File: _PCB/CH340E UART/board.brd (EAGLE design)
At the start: 24.9 x 16.3 mm, 11 parts, among them IC1 REG1117, U1 CH340ESMD

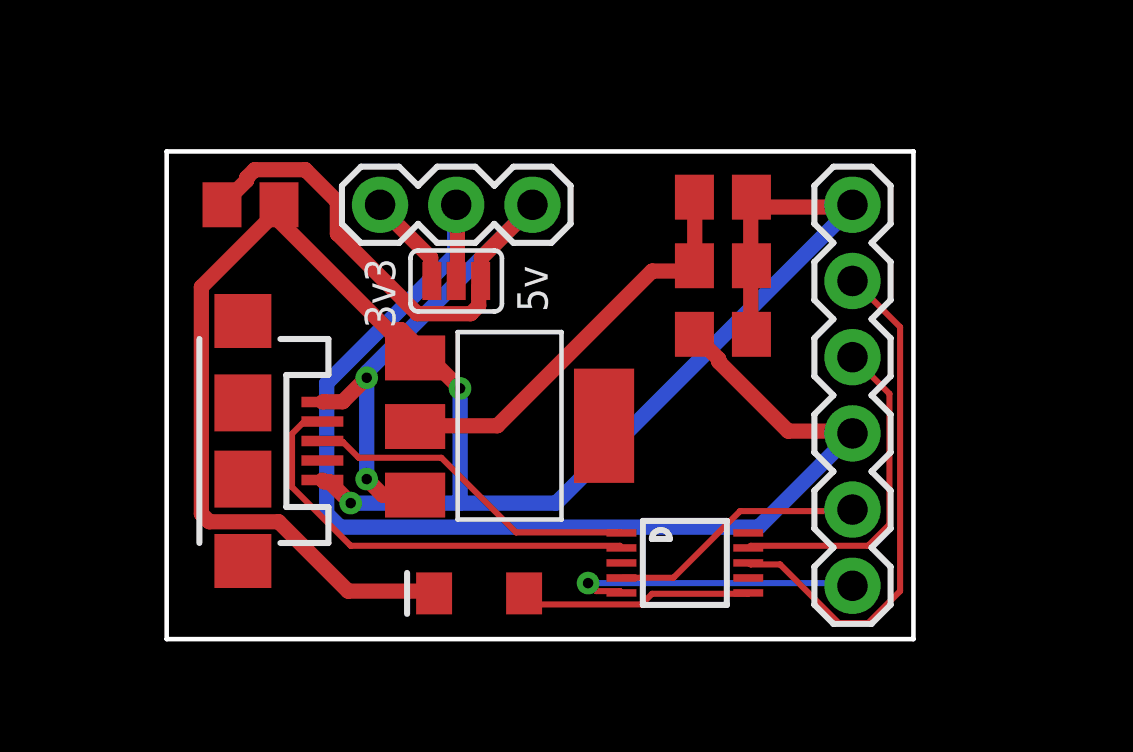
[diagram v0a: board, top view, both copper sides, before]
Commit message: CH340e design complete
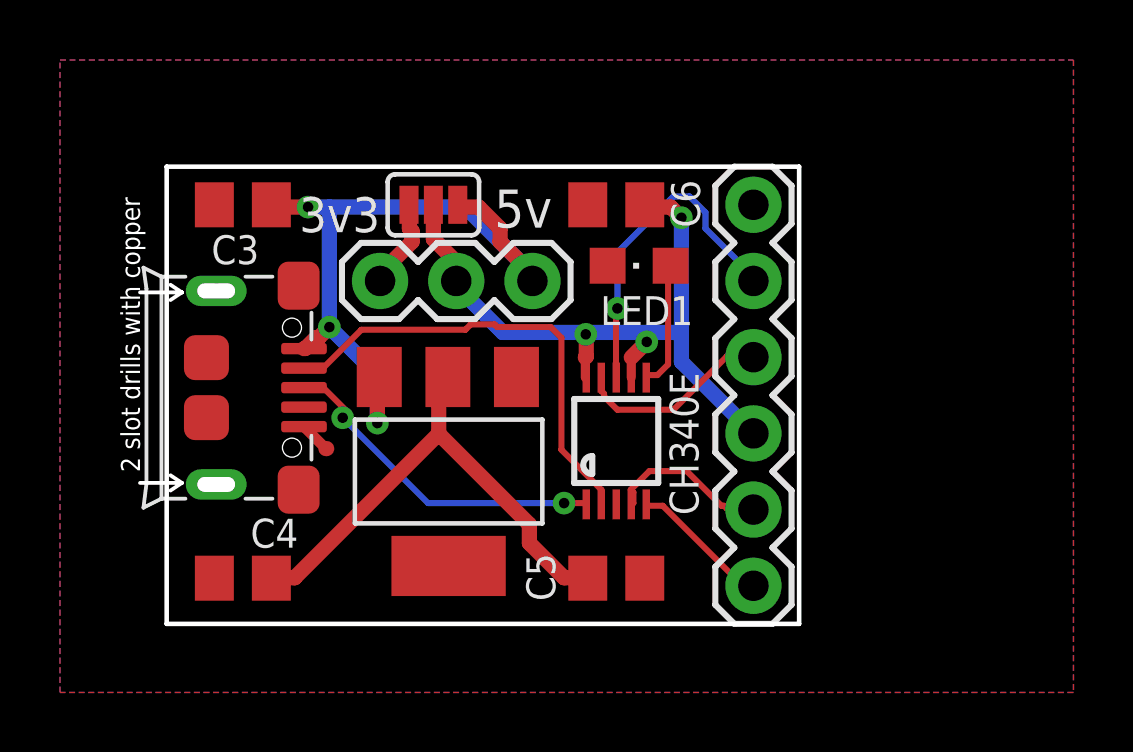
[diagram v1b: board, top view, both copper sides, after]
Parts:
- removed D1: 1206size, SparkFun-LED:LED-1206
- removed J1: (no value), SparkFun-Connectors:USB-MICROB
- removed U1: CH340ESMD, CH340E:MSOP10
- added CH340E: CH340ESMD, CH340E:MSOP10
- added LED1: (no value), adafruit:CHIPLED_0805
- added USB2: ST-USB-001G, Seeed-Connector:MICRO-USB5+4P-SMD-0.65-B
- JP1: device SparkFun-Jumpers:SMT-JUMPER_3_1-NC_PASTE_SILK -> SparkFun-Jumpers:SMT-JUMPER_3_NO_SILK
- moved C4 19.1 mm to (2.54, 2.03), turned to 180 degrees
- moved C5 13.2 mm to (15.0, 2.03)
- moved C6 5.59 mm to (15.0, 14.5), turned to 180 degrees
- moved J2 3.30 mm to (19.6, 1.78)
- moved JP1 2.65 mm to (8.89, 14.5)
- moved IC1 2.54 mm to (9.40, 5.59), turned to 180 degrees
- moved J3 2.54 mm to (12.2, 11.9)
- moved C3 0.25 mm to (2.54, 14.5), turned to 180 degrees
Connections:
- net 5V1 renamed 3V3
- net 5V: now also USB2.1; no longer J1.VBUS
- net CTS: now also CH340E.5; no longer U1.5
- net GND: now also CH340E.3, LED1.C, USB2.5, USB2.S1, USB2.S2, USB2.S3, USB2.S4, USB2.S5, USB2.S6; no longer D1.C, J1.GND, U1.3
- net N$1: now also CH340E.6, LED1.A; no longer D1.A, U1.6
- net RTS: now also CH340E.4; no longer U1.4
- net RX: now also CH340E.9; no longer U1.9
- net TX: now also CH340E.8; no longer U1.8
- net USBN: now also CH340E.2, USB2.2; no longer J1.D-, U1.2
- net USBP: now also CH340E.1, USB2.3; no longer J1.D+, U1.1
- net VCC: now also CH340E.10, CH340E.7; no longer U1.10, U1.7
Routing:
- net GND: track 64.6 -> 1.06 mm, vias 2 -> 0
- net VCC: track 40.4 -> 24.0 mm, vias 0 -> 3
- net 5V: track 31.0 -> 24.4 mm, vias 2 -> 3
- net TX: track 17.3 -> 11.1 mm, vias 0 -> 1
- net CTS: track 10.1 -> 4.71 mm, vias 1 -> 0
- net RX: track 11.1 -> 6.59 mm
- net N$1: track 7.79 -> 4.32 mm
- net RTS: track 8.66 -> 5.47 mm
- net 3V3: track 13.8 -> 16.9 mm
- net USBN: track 14.8 -> 15.5 mm
- net USBP: track 11.2 -> 11.3 mm, vias 0 -> 2
- added copper zone on layer 1, net GND
- added copper zone on layer 16, net GND
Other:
- board size 24.9 x 16.3 mm -> 21.1 x 15.2 mm
- board text added: "CTS"
- board text added: "GND"
- board text added: "RTS"
- board text added: "RX"
- board text added: "TX"
- board text added: "VCC"
